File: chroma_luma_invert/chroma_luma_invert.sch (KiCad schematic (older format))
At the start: 34 parts, among them J1 Barrel_Jack, J2 rca, J3 Conn_01x12, J4 rca, SW1 SPDT, SW2 SPDT, U1 AD8044, U2 LM317, U3 CD4051

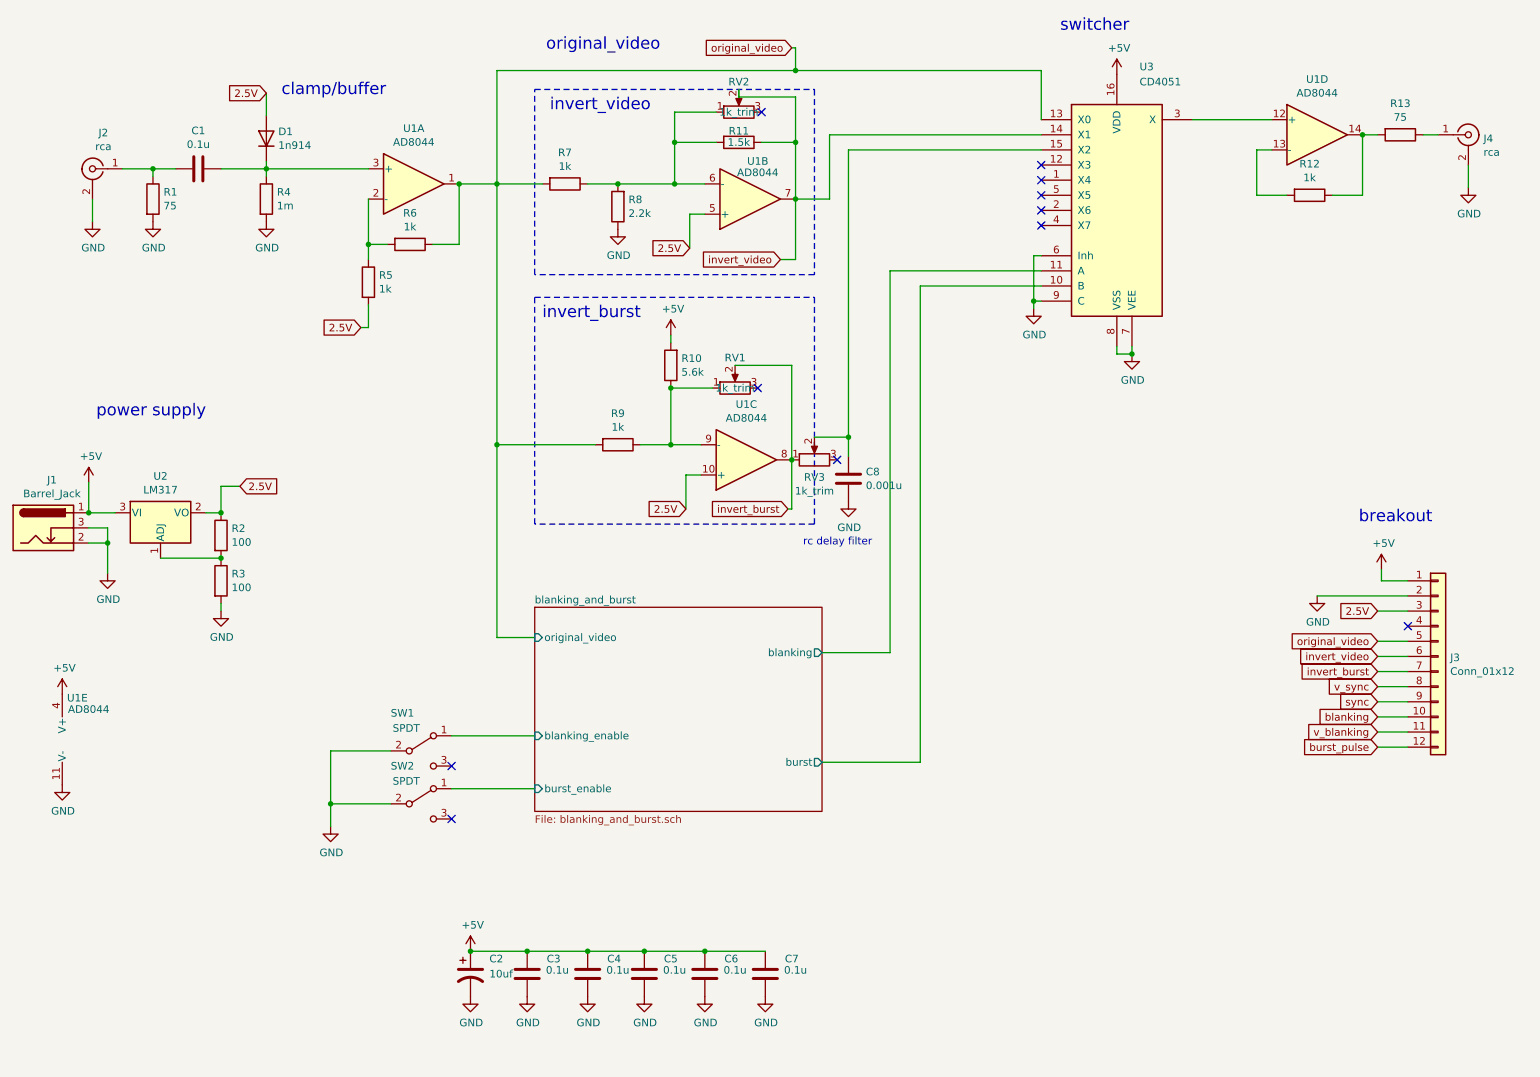
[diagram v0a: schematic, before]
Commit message: working on nexr version for colorizer and inverter
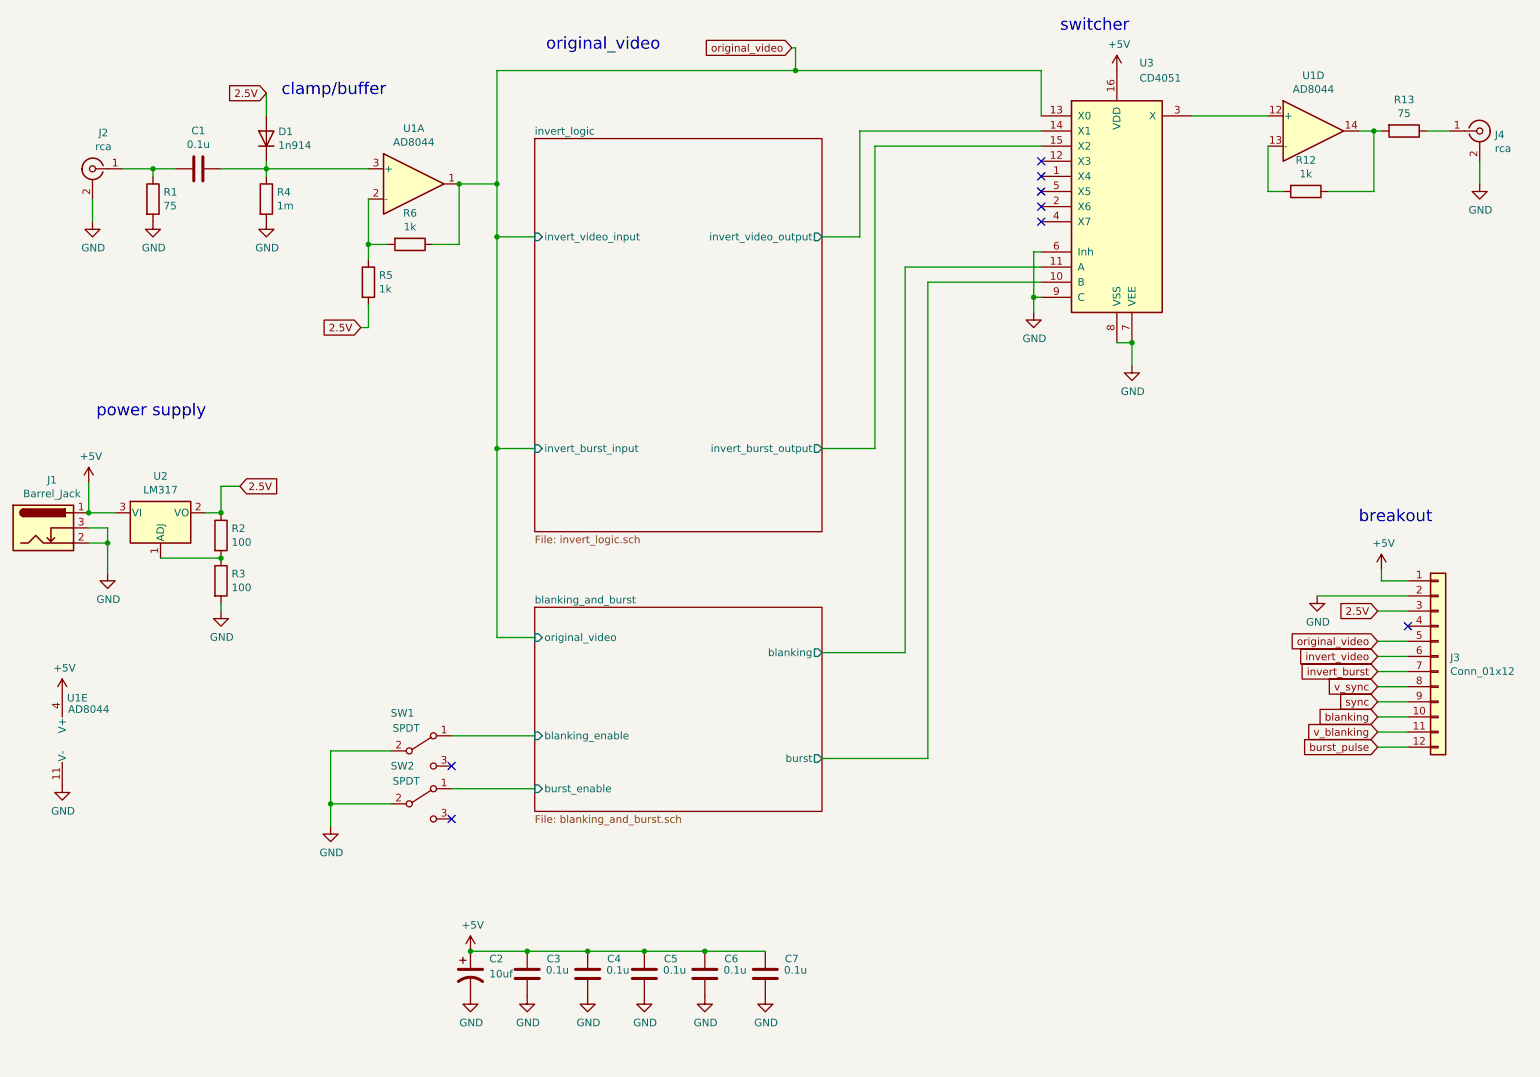
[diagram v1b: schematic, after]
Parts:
- removed C8: 0.001u, Capacitor_THT:C_Disc_D4.7mm_W2.5mm_P5.00mm, symbol Device:C
- removed R10: 5.6k, Resistor_THT:R_Axial_DIN0207_L6.3mm_D2.5mm_P7.62mm_Horizontal, symbol Device:R
- removed R11: 1.5k, Resistor_THT:R_Axial_DIN0207_L6.3mm_D2.5mm_P7.62mm_Horizontal, symbol Device:R
- removed R7, R9: 1k, Resistor_THT:R_Axial_DIN0207_L6.3mm_D2.5mm_P7.62mm_Horizontal, symbol Device:R
- removed R8: 2.2k, Resistor_THT:R_Axial_DIN0207_L6.3mm_D2.5mm_P7.62mm_Horizontal, symbol Device:R
- removed RV1, RV2, RV3: 1k_trim, lib_fp:tht_vertical_trimpot_3362, symbol Device:R_POT
- removed unit 2 of U1
- removed unit 3 of U1
- SW1, SW2: footprint lib_fp:mini_toggle_switch_tayda -> lib_fp:spdt_slide_switch_small_tayda
- U1: footprint project_parts:DIP+SOIC_14 -> lib_fp:DIP+SOIC_14
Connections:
- net invert_video: no longer U3.14 (X1)
- net invert_logic/invert_burst_output: now reaches U3.15 (X2)
- new net invert_logic/invert_video_output: U3.14 (X1)
- no-connect marks 11 -> 8
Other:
- note removed: "invert_burst"
- note removed: "invert_video"
- note removed: "rc delay filter"
- moved on the sheet: J4, R12, R13, U1D, U3

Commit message: newest circuit revisions
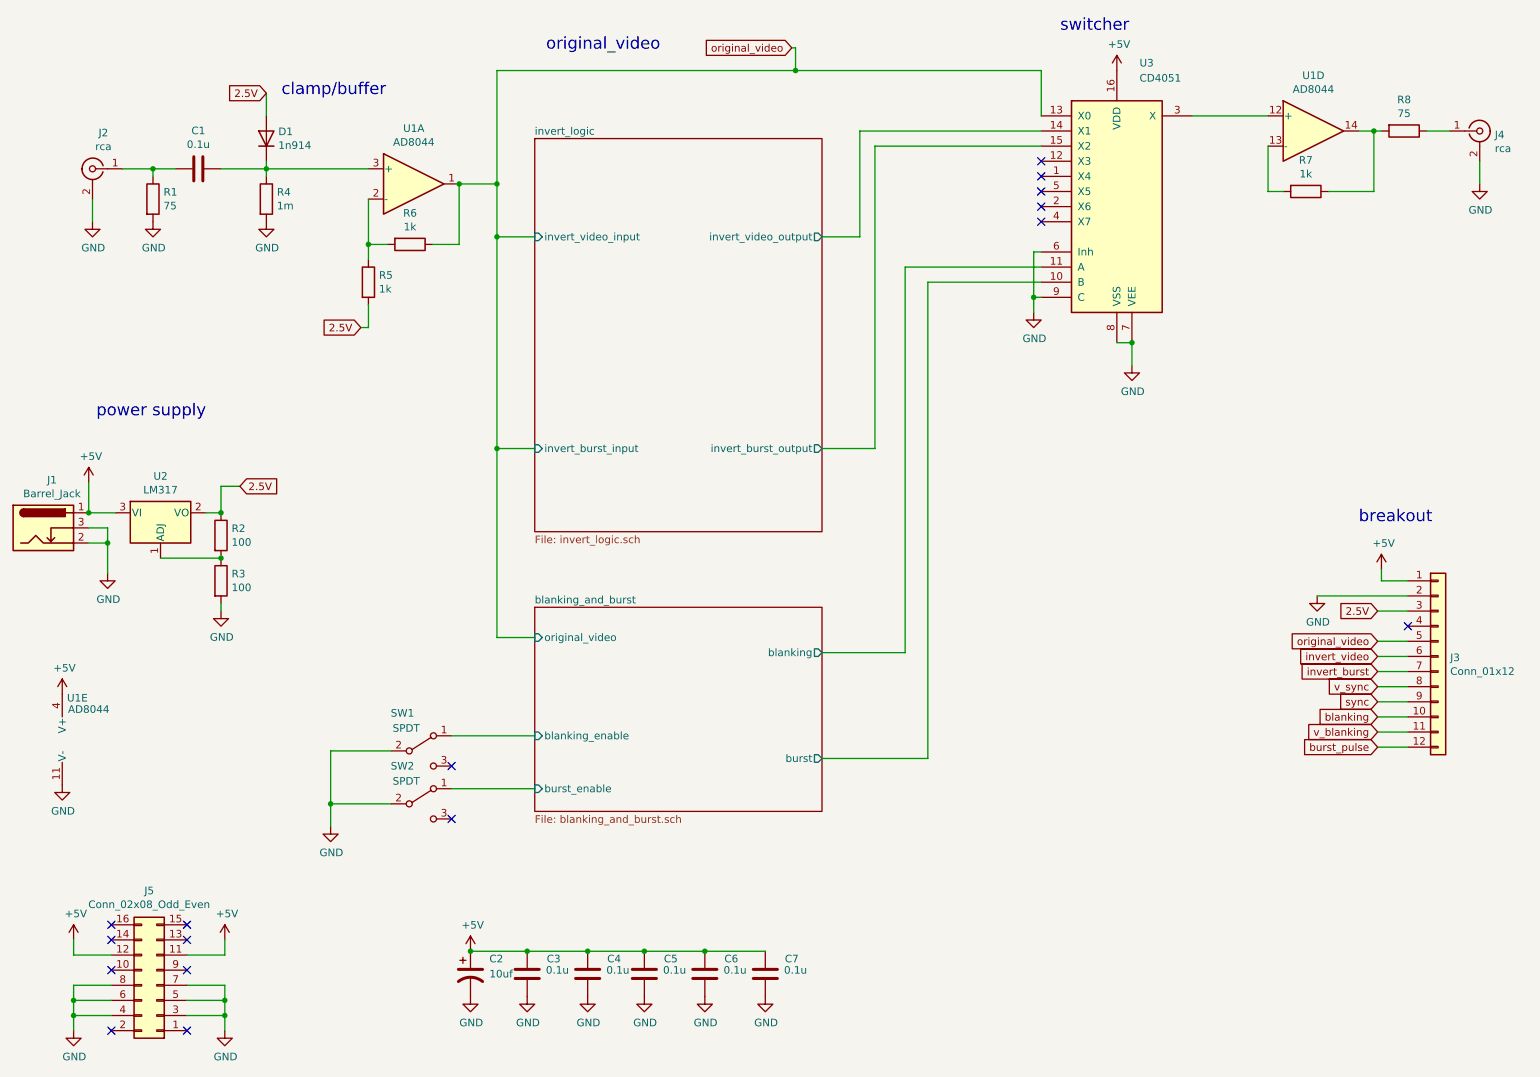
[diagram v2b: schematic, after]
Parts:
- added J5: Conn_02x08_Odd_Even, Connector_PinHeader_2.54mm:PinHeader_2x08_P2.54mm_Vertical, symbol Connector_Generic:Conn_02x08_Odd_Even
- renumbered R12 to R7, R13 to R8
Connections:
- net +5V: now also J5.11 (Pin_11), J5.12 (Pin_12)
- net GND: now also J5.3 (Pin_3), J5.4 (Pin_4), J5.5 (Pin_5), J5.6 (Pin_6), J5.7 (Pin_7), J5.8 (Pin_8)
- no-connect marks 8 -> 16
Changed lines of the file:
@@
 NoConn ~ 7550 1900
 $Comp
-L power:+5V #PWR021
+L power:+5V #PWR018
 U 1 1 5EC0D810
 P 8050 900
-F 0 "#PWR021" H 8050 750 50  0001 C CNN
+F 0 "#PWR018" H 8050 750 50  0001 C CNN
 F 1 "+5V" H 8065 1073 50  0000 C CNN
 F 2 "" H 8050 900 50  0001 C CNN
@@
 $EndComp
 $Comp
-L Device:R R12
+L Device:R R7
 U 1 1 5EC24B54
 P 9300 1700
-F 0 "R12" V 9093 1700 50  0000 C CNN
+F 0 "R7" V 9093 1700 50  0000 C CNN
 F 1 "1k" V 9184 1700 50  0000 C CNN
 F 2 "Resistor_THT:R_Axial_DIN0207_L6.3mm_D2.5mm_P7.62mm_Horizontal" V 9230 1700 50  0001 C CNN
@@
 $EndComp
 $Comp
-L Device:R R13
+L Device:R R8
 U 1 1 5EC26408
 P 9950 1300
-F 0 "R13" V 9743 1300 50  0000 C CNN
+F 0 "R8" V 9743 1300 50  0000 C CNN
 F 1 "75" V 9834 1300 50  0000 C CNN
 F 2 "Resistor_THT:R_Axial_DIN0207_L6.3mm_D2.5mm_P7.62mm_Horizontal" V 9880 1300 50  0001 C CNN
@@
 $EndComp
 $Comp
-L power:GND #PWR025
+L power:GND #PWR022
 U 1 1 5EC28FF2
 P 10450 1650
-F 0 "#PWR025" H 10450 1400 50  0001 C CNN
+F 0 "#PWR022" H 10450 1400 50  0001 C CNN
 F 1 "GND" H 10455 1477 50  0000 C CNN
 F 2 "" H 10450 1650 50  0001 C CNN
@@
 	9975 4475 9775 4475
 $Comp
-L power:+5V #PWR024
+L power:+5V #PWR021
 U 1 1 5ED5EE28
 P 9800 4200
-F 0 "#PWR024" H 9800 4050 50  0001 C CNN
+F 0 "#PWR021" H 9800 4050 50  0001 C CNN
 F 1 "+5V" H 9815 4373 50  0000 C CNN
 F 2 "" H 9800 4200 50  0001 C CNN
@@
 	9800 4275 9800 4200
 $Comp
-L power:GND #PWR023
+L power:GND #PWR020
 U 1 1 5ED61B5B
 P 9375 4375
-F 0 "#PWR023" H 9375 4125 50  0001 C CNN
+F 0 "#PWR020" H 9375 4125 50  0001 C CNN
 F 1 "GND" H 9380 4202 50  0000 C CNN
 F 2 "" H 9375 4375 50  0001 C CNN
@@
 $EndComp
 $Comp
-L power:GND #PWR015
+L power:GND #PWR014
 U 1 1 5F3B3611
 P 4925 7025
-F 0 "#PWR015" H 4925 6775 50  0001 C CNN
+F 0 "#PWR014" H 4925 6775 50  0001 C CNN
 F 1 "GND" H 4930 6852 50  0000 C CNN
 F 2 "" H 4925 7025 50  0001 C CNN
@@
 $EndComp
 $Comp
-L power:GND #PWR017
+L power:GND #PWR015
 U 1 1 5F3B39DD
 P 5325 7025
-F 0 "#PWR017" H 5325 6775 50  0001 C CNN
+F 0 "#PWR015" H 5325 6775 50  0001 C CNN
 F 1 "GND" H 5330 6852 50  0000 C CNN
 F 2 "" H 5325 7025 50  0001 C CNN
@@
 $EndComp
 $Comp
-L power:GND #PWR018
+L power:GND #PWR016
 U 1 1 5F3B3F41
 P 5725 7025
-F 0 "#PWR018" H 5725 6775 50  0001 C CNN
+F 0 "#PWR016" H 5725 6775 50  0001 C CNN
 F 1 "GND" H 5730 6852 50  0000 C CNN
 F 2 "" H 5725 7025 50  0001 C CNN
@@
 	6450 1400 7550 1400
 $Comp
-L power:GND #PWR020
+L power:GND #PWR017
 U 1 1 5EC1216C
 P 7500 2500
-F 0 "#PWR020" H 7500 2250 50  0001 C CNN
+F 0 "#PWR017" H 7500 2250 50  0001 C CNN
 F 1 "GND" H 7505 2327 50  0000 C CNN
 F 2 "" H 7500 2500 50  0001 C CNN
@@
 	7550 1200 7550 900
 $Comp
-L power:GND #PWR014
+L power:GND #PWR019
 U 1 1 61B4819B
 P 8150 2850
-F 0 "#PWR014" H 8150 2600 50  0001 C CNN
+F 0 "#PWR019" H 8150 2600 50  0001 C CNN
 F 1 "GND" H 8155 2677 50  0000 C CNN
 F 2 "" H 8150 2850 50  0001 C CNN
@@
 Wire Wire Line
 	3950 3400 3950 4650
+$Comp
+L Connector_Generic:Conn_02x08_Odd_Even J5
+U 1 1 6167F829
+P 1700 6950
+F 0 "J5" H 1750 6325 50  0000 C CNN
+F 1 "Conn_02x08_Odd_Even" H 1750 6416 50  0000 C CNN
+F 2 "Connector_PinHeader_2.54mm:PinHeader_2x08_P2.54mm_Vertical" H 1700 6950 50  0001 C CNN
+F 3 "~" H 1700 6950 50  0001 C CNN
+	1    1700 6950
+	-1   0    0    1
+$EndComp
+$Comp
+L power:GND #PWR0101
+U 1 1 6168109E
+P 2150 7250
+F 0 "#PWR0101" H 2150 7000 50  0001 C CNN
+F 1 "GND" H 2155 7077 50  0000 C CNN
+F 2 "" H 2150 7250 50  0001 C CNN
+F 3 "" H 2150 7250 50  0001 C CNN
+	1    2150 7250
+	1    0    0    -1
+$EndComp
+Wire Wire Line
+	1900 6950 2150 6950
+Wire Wire Line
+	2150 6950 2150 7050
+Wire Wire Line
+	1900 7150 2150 7150
+Connection ~ 2150 7150
+Wire Wire Line
+	2150 7150 2150 7250
+Wire Wire Line
+	1900 7050 2150 7050
+Connection ~ 2150 7050
+Wire Wire Line
+	2150 7050 2150 7150
+$Comp
+L power:GND #PWR0102
+U 1 1 616890ED
+P 1150 7250
+F 0 "#PWR0102" H 1150 7000 50  0001 C CNN
+F 1 "GND" H 1155 7077 50  0000 C CNN
+F 2 "" H 1150 7250 50  0001 C CNN
+F 3 "" H 1150 7250 50  0001 C CNN
+	1    1150 7250
+	1    0    0    -1
+$EndComp
+Wire Wire Line
+	1150 7250 1150 7150
+Wire Wire Line
+	1150 7150 1400 7150
+Wire Wire Line
+	1150 7150 1150 7050
+Wire Wire Line
+	1150 7050 1400 7050
+Connection ~ 1150 7150
+Wire Wire Line
+	1150 7050 1150 6950
+Wire Wire Line
+	1150 6950 1400 6950
+Connection ~ 1150 7050
+$Comp
+L power:+5V #PWR0103
+U 1 1 616AC00F
+P 1150 6650
+F 0 "#PWR0103" H 1150 6500 50  0001 C CNN
+F 1 "+5V" H 1165 6823 50  0000 C CNN
+F 2 "" H 1150 6650 50  0001 C CNN
+F 3 "" H 1150 6650 50  0001 C CNN
+	1    1150 6650
+	1    0    0    -1
+$EndComp
+Wire Wire Line
+	1150 6750 1400 6750
+Wire Wire Line
+	1150 6650 1150 6750
+$Comp
+L power:+5V #PWR0104
+U 1 1 616B447D
+P 2150 6650
+F 0 "#PWR0104" H 2150 6500 50  0001 C CNN
+F 1 "+5V" H 2165 6823 50  0000 C CNN
+F 2 "" H 2150 6650 50  0001 C CNN
+F 3 "" H 2150 6650 50  0001 C CNN
+	1    2150 6650
+	1    0    0    -1
+$EndComp
+Wire Wire Line
+	2150 6650 2150 6750
+Wire Wire Line
+	2150 6750 1900 6750
+NoConn ~ 1400 6550
+NoConn ~ 1400 6650
+NoConn ~ 1900 6550
+NoConn ~ 1900 6650
+NoConn ~ 1400 6850
+NoConn ~ 1900 6850
+NoConn ~ 1400 7250
+NoConn ~ 1900 7250
 $EndSCHEMATC
